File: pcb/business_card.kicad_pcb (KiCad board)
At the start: 2 copper layers, 88.9 x 50.8 mm, 71 parts, among them J3 USB_A, J4 Conn_ARM_SWD_TagConnect_TC2030, SW1 SW_SPST, U1 MIC5504-3.3YM5, U2 STM32G030F6P6

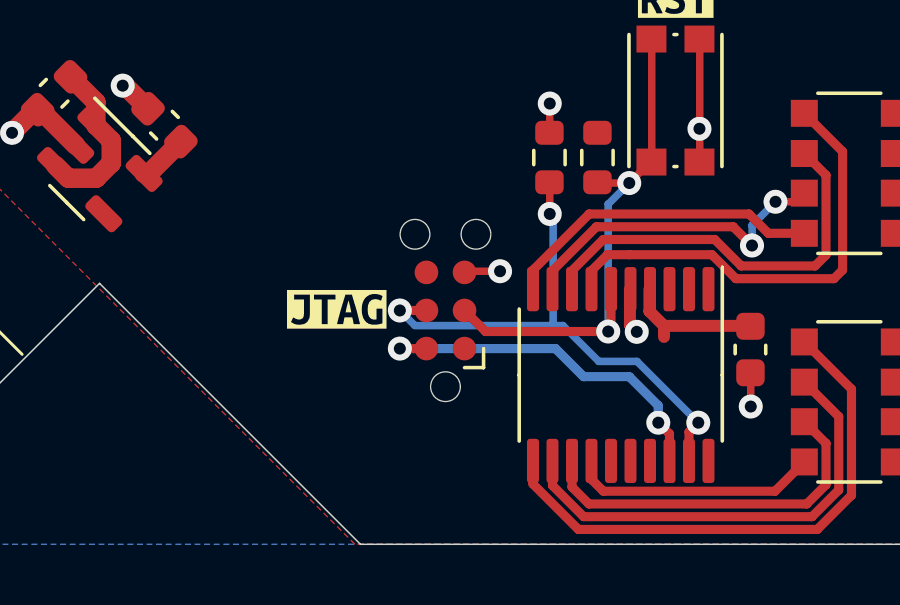
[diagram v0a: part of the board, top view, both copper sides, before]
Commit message: add updates
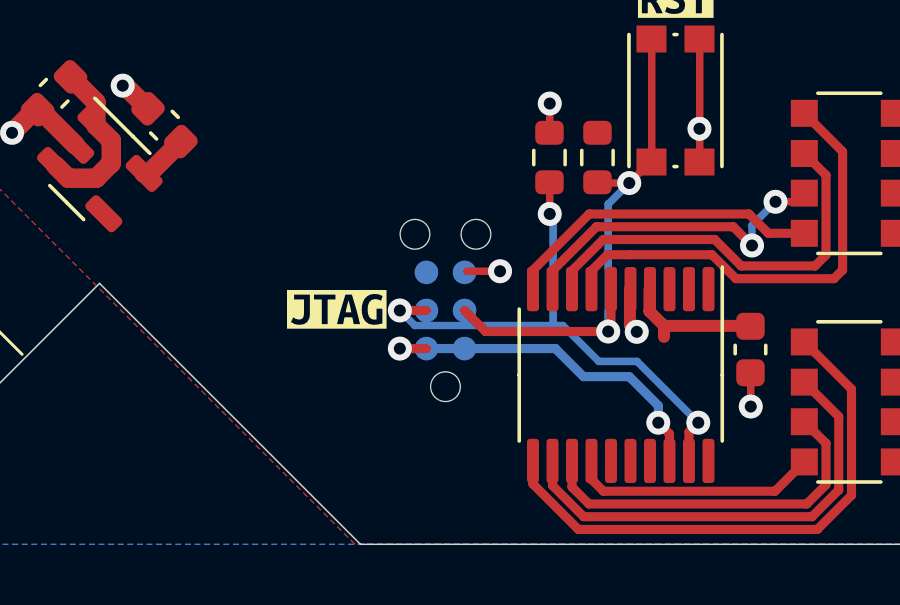
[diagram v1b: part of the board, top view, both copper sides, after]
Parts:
- J4: moved to B.Cu
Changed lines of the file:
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@@
-    )
-  )
-  (footprint "Connector:Tag-Connect_TC2030-IDC-NL_2x03_P1.27mm_Vertical" (layer "F.Cu")
-    (at 127.985796 121.746296 90)
-    (descr "Tag-Connect programming header; http://www.tag-connect.com/Materials/TC2030-IDC-NL.pdf")
-    (tags "tag connect programming header pogo pins")
-    (property "Sheetfile" "business_card_v1.kicad_sch")
-    (property "Sheetname" "")
-    (property "exclude_from_bom" "")
-    (property "ki_description" "Tag-Connect ARM Cortex SWD JTAG connector, 6 pin")
-    (property "ki_keywords" "Cortex Debug Connector ARM SWD JTAG")
-    (attr exclude_from_pos_files exclude_from_bom)
-    (fp_text reference "J4" (at 0 2.7 90) (layer "F.SilkS") hide
-        (effects (font (size 1 1) (thickness 0.15)))
-    )
-    (fp_text value "Conn_ARM_SWD_TagConnect_TC2030" (at 0 -2.3 90) (layer "F.Fab") hide
-        (effects (font (size 1 1) (thickness 0.15)))
-    )
-    (fp_text user "KEEPOUT" (at 0 0 90) (layer "Cmts.User") hide
-        (effects (font (size 0.4 0.4) (thickness 0.07)))
-    )
-    (fp_text user "${REFERENCE}" (at 0 0 90) (layer "F.Fab")
-        (effects (font (size 1 1) (thickness 0.15)))
-    )
-    (fp_line (start -1.905 1.27) (end -1.905 0.635)
-      (stroke (width 0.12) (type solid)) (layer "F.SilkS"))
-    (fp_line (start -1.27 1.27) (end -1.905 1.27)
-      (stroke (width 0.12) (type solid)) (layer "F.SilkS"))
-    (fp_line (start -3.5 -2) (end 3.5 -2)
-      (stroke (width 0.05) (type solid)) (layer "F.CrtYd"))
-    (fp_line (start -3.5 2) (end -3.5 -2)
-      (stroke (width 0.05) (type solid)) (layer "F.CrtYd"))
-    (fp_line (start 3.5 -2) (end 3.5 2)
-      (stroke (width 0.05) (type solid)) (layer "F.CrtYd"))
-    (fp_line (start 3.5 2) (end -3.5 2)
-      (stroke (width 0.05) (type solid)) (layer "F.CrtYd"))
-    (pad "" np_thru_hole circle (at -2.54 0 90) (size 0.9906 0.9906) (drill 0.9906) (layers "*.Cu" "*.Mask"))
-    (pad "" np_thru_hole circle (at 2.54 -1.016 90) (size 0.9906 0.9906) (drill 0.9906) (layers "*.Cu" "*.Mask"))
-    (pad "" np_thru_hole circle (at 2.54 1.016 90) (size 0.9906 0.9906) (drill 0.9906) (layers "*.Cu" "*.Mask"))
-    (pad "1" connect circle (at -1.27 0.635 90) (size 0.7874 0.7874) (layers "F.Cu" "F.Mask")
-      (net 6 "+3V3") (pinfunction "VCC") (pintype "power_in"))
-    (pad "2" connect circle (at -1.27 -0.635 90) (size 0.7874 0.7874) (layers "F.Cu" "F.Mask")
-      (net 7 "SWDIO") (pinfunction "SWDIO") (pintype "bidirectional"))
-    (pad "3" connect circle (at 0 0.635 90) (size 0.7874 0.7874) (layers "F.Cu" "F.Mask")
-      (net 2 "~{RST}") (pinfunction "~{RESET}") (pintype "open_collector"))
-    (pad "4" connect circle (at 0 -0.635 90) (size 0.7874 0.7874) (layers "F.Cu" "F.Mask")
-      (net 3 "SWDCLK") (pinfunction "SWCLK") (pintype "output"))
-    (pad "5" connect circle (at 1.27 0.635 90) (size 0.7874 0.7874) (layers "F.Cu" "F.Mask")
-      (net 1 "GND") (pinfunction "GND") (pintype "power_in"))
-    (pad "6" connect circle (at 1.27 -0.635 90) (size 0.7874 0.7874) (layers "F.Cu" "F.Mask")
-      (net 4 "unconnected-(J4-SWO-Pad6)") (pinfunction "SWO") (pintype "input+no_connect"))
-    (zone (net 0) (net_name "") (layer "F.Cu") (hatch full 0.508)
-      (connect_pads (clearance 0))
-      (min_thickness 0.254) (filled_areas_thickness no)
-      (keepout (tracks allowed) (vias not_allowed) (pads allowed) (copperpour not_allowed) (footprints not_allowed))
-      (fill (thermal_gap 0.508) (thermal_bridge_width 0.508))
-      (polygon
-        (pts
-          (xy 127.350796 120.476296)
-          (xy 127.350796 123.016296)
-          (xy 128.620796 123.016296)
-          (xy 128.620796 120.476296)
-        )
-      )
     )
   )
@@
     )
   )
+  (footprint "Connector:Tag-Connect_TC2030-IDC-NL_2x03_P1.27mm_Vertical" (layer "B.Cu")
+    (at 127.985796 121.746296 90)
+    (descr "Tag-Connect programming header; http://www.tag-connect.com/Materials/TC2030-IDC-NL.pdf")
+    (tags "tag connect programming header pogo pins")
+    (property "Sheetfile" "business_card_v1.kicad_sch")
+    (property "Sheetname" "")
+    (property "exclude_from_bom" "")
+    (property "ki_description" "Tag-Connect ARM Cortex SWD JTAG connector, 6 pin")
+    (property "ki_keywords" "Cortex Debug Connector ARM SWD JTAG")
+    (attr exclude_from_pos_files exclude_from_bom)
+    (fp_text reference "J4" (at 0 -2.7 90) (layer "B.SilkS") hide
+        (effects (font (size 1 1) (thickness 0.15)) (justify mirror))
+    )
+    (fp_text value "Conn_ARM_SWD_TagConnect_TC2030" (at 0 2.3 90) (layer "B.Fab") hide
+        (effects (font (size 1 1) (thickness 0.15)) (justify mirror))
+    )
+    (fp_text user "KEEPOUT" (at 0 0 90) (layer "Cmts.User") hide
+        (effects (font (size 0.4 0.4) (thickness 0.07)))
+    )
+    (fp_text user "${REFERENCE}" (at 0 0 90) (layer "B.Fab")
+        (effects (font (size 1 1) (thickness 0.15)) (justify mirror))
+    )
+    (fp_line (start -1.905 -1.27) (end -1.905 -0.635)
+      (stroke (width 0.12) (type solid)) (layer "B.SilkS"))
+    (fp_line (start -1.27 -1.27) (end -1.905 -1.27)
+      (stroke (width 0.12) (type solid)) (layer "B.SilkS"))
+    (fp_line (start -3.5 -2) (end -3.5 2)
+      (stroke (width 0.05) (type solid)) (layer "B.CrtYd"))
+    (fp_line (start -3.5 2) (end 3.5 2)
+      (stroke (width 0.05) (type solid)) (layer "B.CrtYd"))
+    (fp_line (start 3.5 -2) (end -3.5 -2)
+      (stroke (width 0.05) (type solid)) (layer "B.CrtYd"))
+    (fp_line (start 3.5 2) (end 3.5 -2)
+      (stroke (width 0.05) (type solid)) (layer "B.CrtYd"))
+    (pad "" np_thru_hole circle (at -2.54 0 90) (size 0.9906 0.9906) (drill 0.9906) (layers "*.Cu" "*.Mask"))
+    (pad "" np_thru_hole circle (at 2.54 -1.016 90) (size 0.9906 0.9906) (drill 0.9906) (layers "*.Cu" "*.Mask"))
+    (pad "" np_thru_hole circle (at 2.54 1.016 90) (size 0.9906 0.9906) (drill 0.9906) (layers "*.Cu" "*.Mask"))
+    (pad "1" connect circle (at -1.27 -0.635 90) (size 0.7874 0.7874) (layers "B.Cu" "B.Mask")
+      (net 6 "+3V3") (pinfunction "VCC") (pintype "power_in"))
+    (pad "2" connect circle (at -1.27 0.635 90) (size 0.7874 0.7874) (layers "B.Cu" "B.Mask")
+      (net 7 "SWDIO") (pinfunction "SWDIO") (pintype "bidirectional"))
+    (pad "3" connect circle (at 0 -0.635 90) (size 0.7874 0.7874) (layers "B.Cu" "B.Mask")
+      (net 2 "~{RST}") (pinfunction "~{RESET}") (pintype "open_collector"))
+    (pad "4" connect circle (at 0 0.635 90) (size 0.7874 0.7874) (layers "B.Cu" "B.Mask")
+      (net 3 "SWDCLK") (pinfunction "SWCLK") (pintype "output"))
+    (pad "5" connect circle (at 1.27 -0.635 90) (size 0.7874 0.7874) (layers "B.Cu" "B.Mask")
+      (net 1 "GND") (pinfunction "GND") (pintype "power_in"))
+    (pad "6" connect circle (at 1.27 0.635 90) (size 0.7874 0.7874) (layers "B.Cu" "B.Mask")
+      (net 4 "unconnected-(J4-SWO-Pad6)") (pinfunction "SWO") (pintype "input+no_connect"))
+    (zone (net 0) (net_name "") (layer "B.Cu") (hatch full 0.508)
+      (connect_pads (clearance 0))
+      (min_thickness 0.254) (filled_areas_thickness no)
+      (keepout (tracks allowed) (vias not_allowed) (pads allowed) (copperpour not_allowed) (footprints not_allowed))
+      (fill (thermal_gap 0.508) (thermal_bridge_width 0.508))
+      (polygon
+        (pts
+          (xy 128.620796 120.476296)
+          (xy 128.620796 123.016296)
+          (xy 127.350796 123.016296)
+          (xy 127.350796 120.476296)
+        )
+      )
+    )
+  )
